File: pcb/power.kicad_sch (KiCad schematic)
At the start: 8 parts, among them U4 LP3993-33B3F

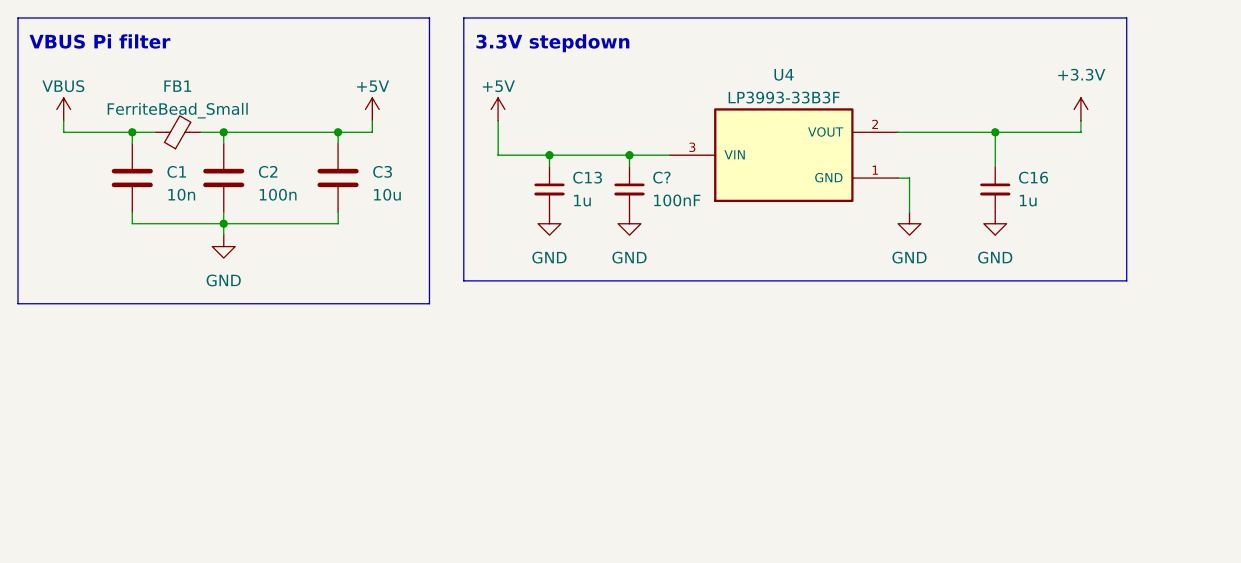
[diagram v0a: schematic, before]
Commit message: PCB work in progress
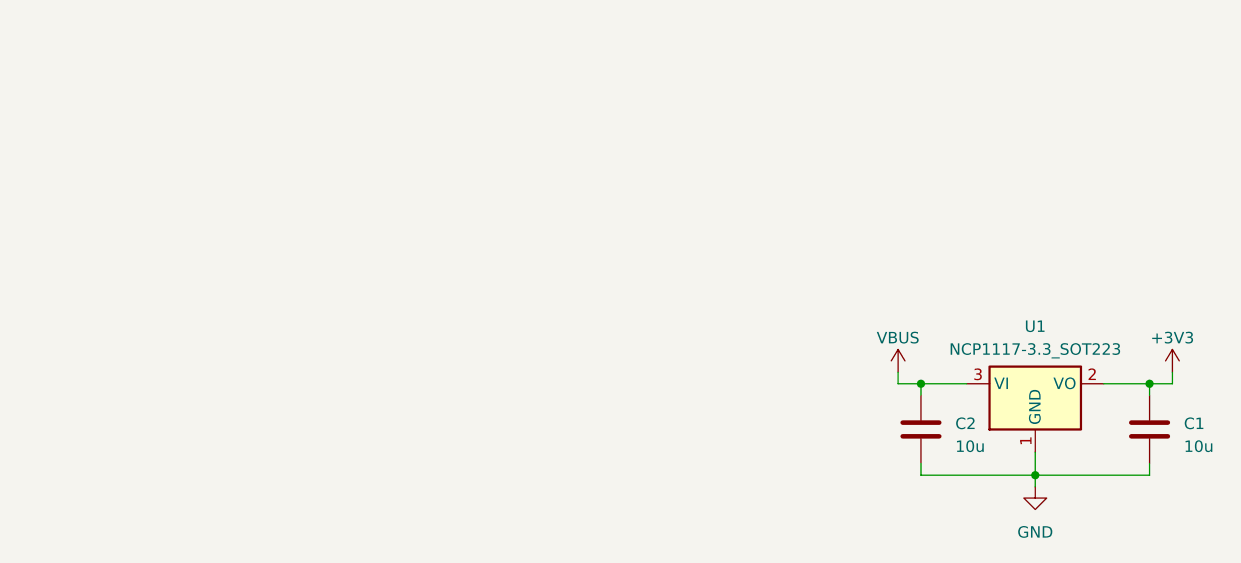
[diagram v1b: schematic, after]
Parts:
- removed C13, C16: 1u, Capacitor_SMD:C_0603_1608Metric, symbol Device:C_Small
- removed C3: 10u, Capacitor_SMD:C_0805_2012Metric, symbol Device:C
- removed C?: 100nF, Capacitor_SMD:C_0603_1608Metric, symbol Device:C_Small
- removed FB1: FerriteBead_Small, Inductor_SMD:L_0603_1608Metric, symbol Device:FerriteBead_Small
- removed U4: LP3993-33B3F, Package_TO_SOT_SMD:SOT-23, symbol AP2210N-3.3TRG1:AP2210N-3.3TRG1
- added U1: NCP1117-3.3_SOT223, Package_TO_SOT_SMD:SOT-223-3_TabPin2, symbol Regulator_Linear:NCP1117-3.3_SOT223
- C1: value 10n -> 10u; footprint Capacitor_SMD:C_0603_1608Metric -> Capacitor_SMD:C_0603_1608Metric_Pad1.08x0.95mm_HandSolder
- C2: value 100n -> 10u; footprint Capacitor_SMD:C_0603_1608Metric -> Capacitor_SMD:C_0603_1608Metric_Pad1.08x0.95mm_HandSolder
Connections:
- net +5V is gone; now on net VBUS: C2.1
- net GND: now also U1.1 (GND)
- net VBUS: now also U1.3 (VI); no longer C1.1
- new net +3V3: C1.1, U1.2 (VO)
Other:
- note removed: "3.3V stepdown"
- note removed: "VBUS Pi filter"
